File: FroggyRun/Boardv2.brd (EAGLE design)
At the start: 18 parts

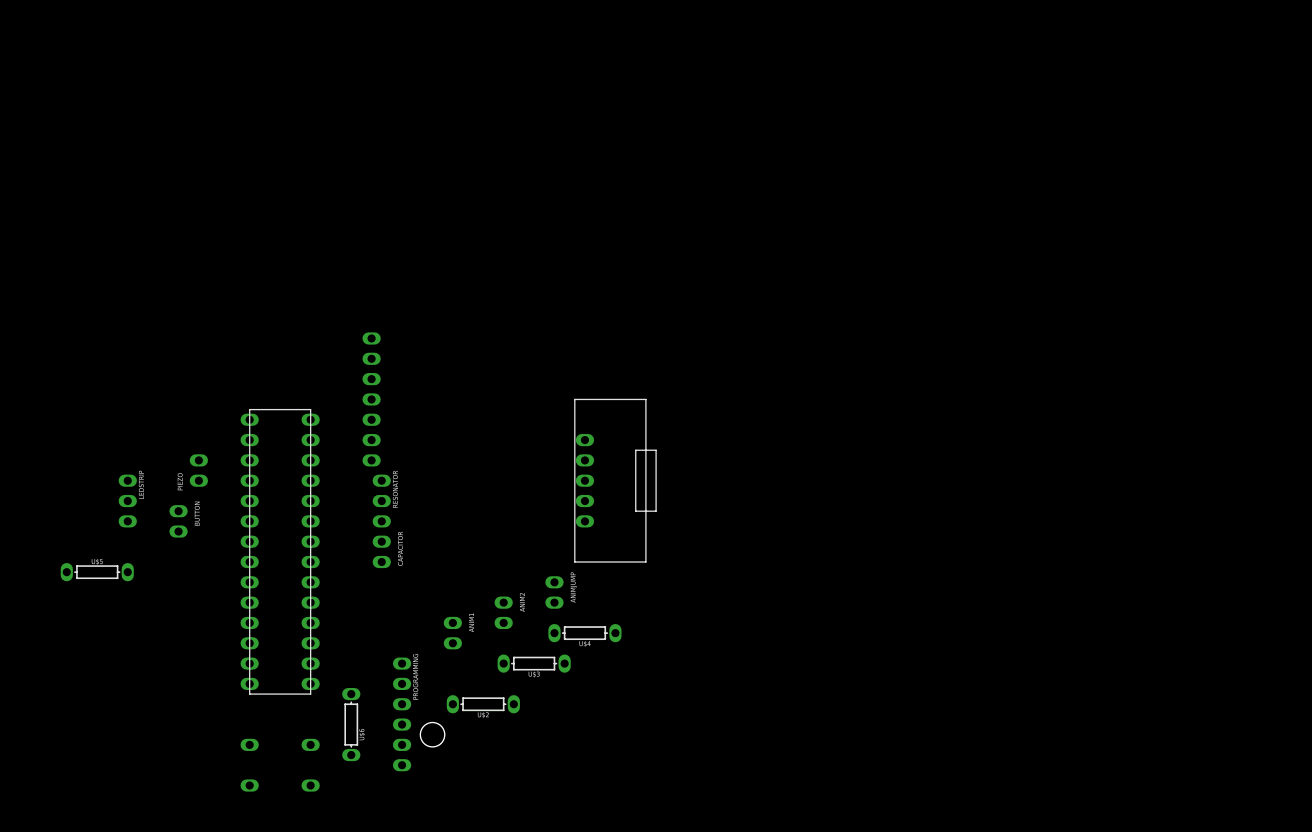
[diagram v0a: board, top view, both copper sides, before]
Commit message: ghkj
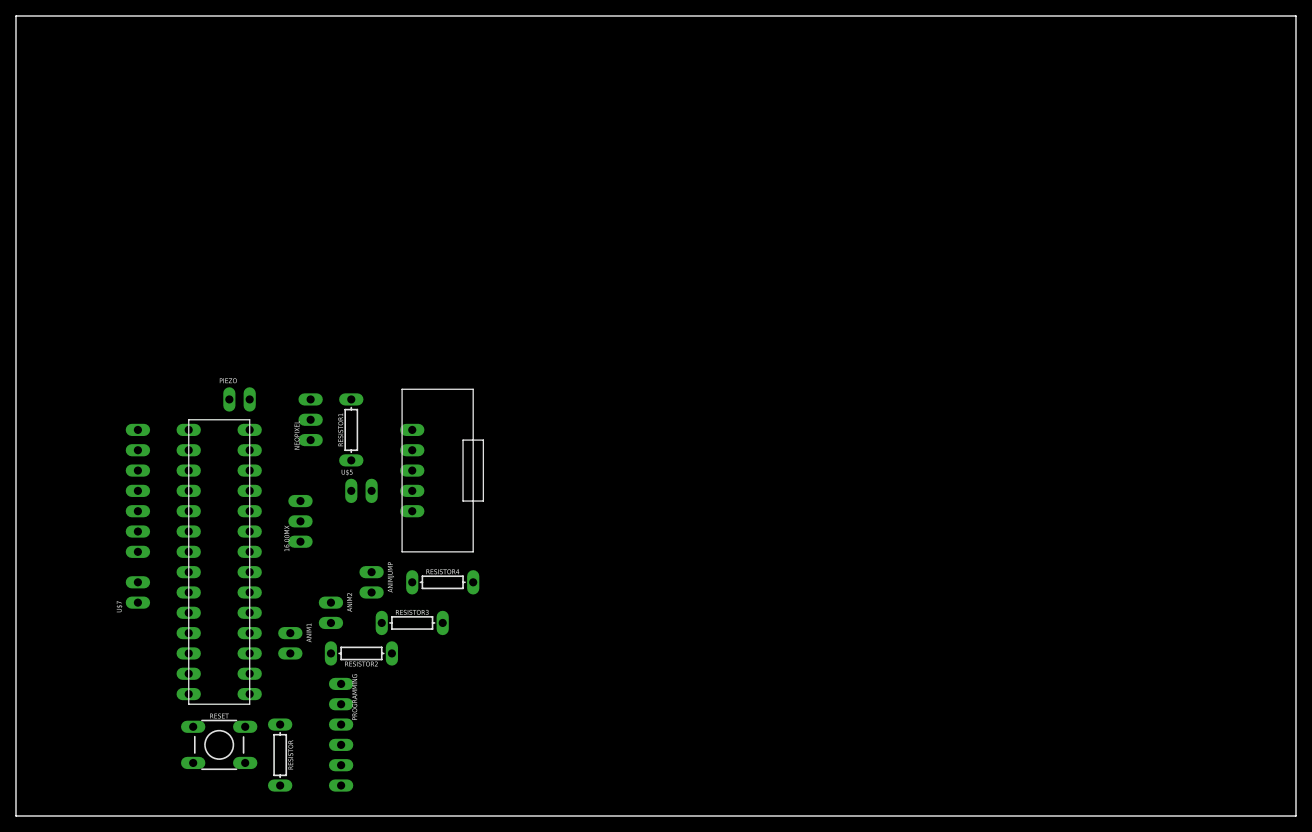
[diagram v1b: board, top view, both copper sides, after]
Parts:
- removed BUTTON, CAPACITOR: 1X2, FroggyRun:1X02_LONGPADS
- removed LEDSTRIP, RESONATOR: 1X3, FroggyRun:1X03_NO_SILK
- removed OLED: OLED, FroggyRun:OLED
- removed U$3, U$4: 1k, FroggyRun:AXIAL-0.3
- removed U$8: USB, FroggyRun:USB
- added 16.00MX: RESONATOR, FroggyRun:1X03_NO_SILK
- added NEOPIXEL: 1X3, FroggyRun:1X03_NO_SILK
- added RESET: MOMENTARY_SWITCH, FroggyRun:TACTILE_SWITCH_PTH_6.0MM
- added RESISTOR, RESISTOR1: 10k, FroggyRun:AXIAL-0.3
- added RESISTOR2, RESISTOR3, RESISTOR4: 470, FroggyRun:AXIAL-0.3
- ANIM1, ANIM2, ANIMJUMP: value 1X2 -> LED
- U$2: value 1k -> USB; device FroggyRun:AXIAL-0.3 -> FroggyRun:USB
- U$5: value 1k -> BUTTON(OFFBOARD); device FroggyRun:AXIAL-0.3 -> FroggyRun:1X02_LONGPADS
- U$6: value 1k -> OLED; device FroggyRun:AXIAL-0.3 -> FroggyRun:OLED
- U$7: value BUTTON -> CAPACITOR; device FroggyRun:BUTTON -> FroggyRun:1X02_LONGPADS
- moved U$6 48.0 mm to (12.7, 49.5)
- moved U$5 33.3 mm to (41.9, 40.6)
- moved U$7 31.4 mm to (15.2, 26.7)
- moved U$2 29.9 mm to (52.1, 43.2), turned to 270 degrees
- moved ANIMJUMP 22.9 mm to (44.5, 30.5)
- moved ANIM2 21.6 mm to (39.4, 26.7)
- moved ANIM1 20.4 mm to (34.3, 22.9)
- moved PIEZO 10.9 mm to (26.7, 52.1), turned to 0 degrees
- moved PROGRAMMING 8.03 mm to (40.6, 16.5)
- moved U$1 7.73 mm to (30.5, 14.0)
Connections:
- net N$12 renamed ANIM1
- net N$13 renamed ANIM2
- net N$14 renamed ANIMJUMP
- net N$17 renamed PROGRAMMING
- removed net N$15: U$1.1, U$6.P$1, U$7.P$2
- removed net N$18: RESONATOR.3, U$1.9
- removed net N$19: RESONATOR.1, U$1.10
- removed net N$20: CAPACITOR.1, U$1.8, U$8.GND
- removed net N$21: CAPACITOR.2, U$1.7, U$8.5V
- removed net N$3 (its old number): OLED.DATA, U$1.12
- removed net VIN: BUTTON.2, LEDSTRIP.3, OLED.VIN, PROGRAMMING.4, U$1.20, U$6.P$2
- new net 5V: NEOPIXEL.1, PROGRAMMING.4, RESET.1, RESET.3, U$1.20, U$1.7, U$2.5V, U$5.2, U$6.VIN, U$7.1
- new net N$12: U$1.19, U$6.RST
- new net NEOPIXEL: NEOPIXEL.2, U$1.12
- new net PIEZO: PIEZO.1, U$1.13
- new net RESET: RESET.2, RESET.4, RESISTOR.P$1, U$1.1
- net GND: now also 16.00MX.2, NEOPIXEL.3, PIEZO.2, RESISTOR.P$2, RESISTOR1.P$2, RESISTOR2.P$2, RESISTOR3.P$2, RESISTOR4.P$2, U$1.21, U$1.8, U$2.GND, U$6.GND, U$7.2; no longer LEDSTRIP.1, OLED.GND, PIEZO.1, RESONATOR.2, U$1.22, U$2.P$1, U$3.P$1, U$4.P$1, U$5.P$1, U$7.P$1
- net N$1: now also ANIM1.2, RESISTOR2.P$1; no longer BUTTON.1, U$1.19, U$5.P$2
- net N$10: now also U$1.17, U$6.SA0; no longer ANIM2.2, U$3.P$2
- net N$11: now also U$1.18, U$6.CS; no longer ANIMJUMP.2, U$4.P$2
- net N$2: now also ANIM2.2, RESISTOR3.P$1; no longer LEDSTRIP.2, U$1.18
- net N$4: now also ANIMJUMP.2, RESISTOR4.P$1; no longer OLED.CLK, U$1.13
- net N$5: now also RESISTOR1.P$1, U$1.11, U$5.1; no longer OLED.SA0, U$1.14
- net N$6: now also 16.00MX.1, U$1.9; no longer OLED.CS, U$1.15
- net N$7: now also 16.00MX.3, U$1.10; no longer OLED.RST, U$1.16
- net N$8: now also U$1.15, U$6.DATA; no longer PIEZO.2, U$1.17
- net N$9: now also U$1.16, U$6.CLK; no longer ANIM1.2, U$2.P$2
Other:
- board outline added: 160 x 100 mm
